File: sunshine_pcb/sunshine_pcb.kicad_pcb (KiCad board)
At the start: 4 copper layers, 30.5 x 44.7 mm, 51 parts, among them J1 VSENS, J2 Conn_01x04, J5 VerticalUSB, Q1 AO3400A, U1 ESP32-S3-WROOM-1, U2 SPX1117M3, U3 LIS3MDL, U4 ADXL375, U8 USBLC6-2P6

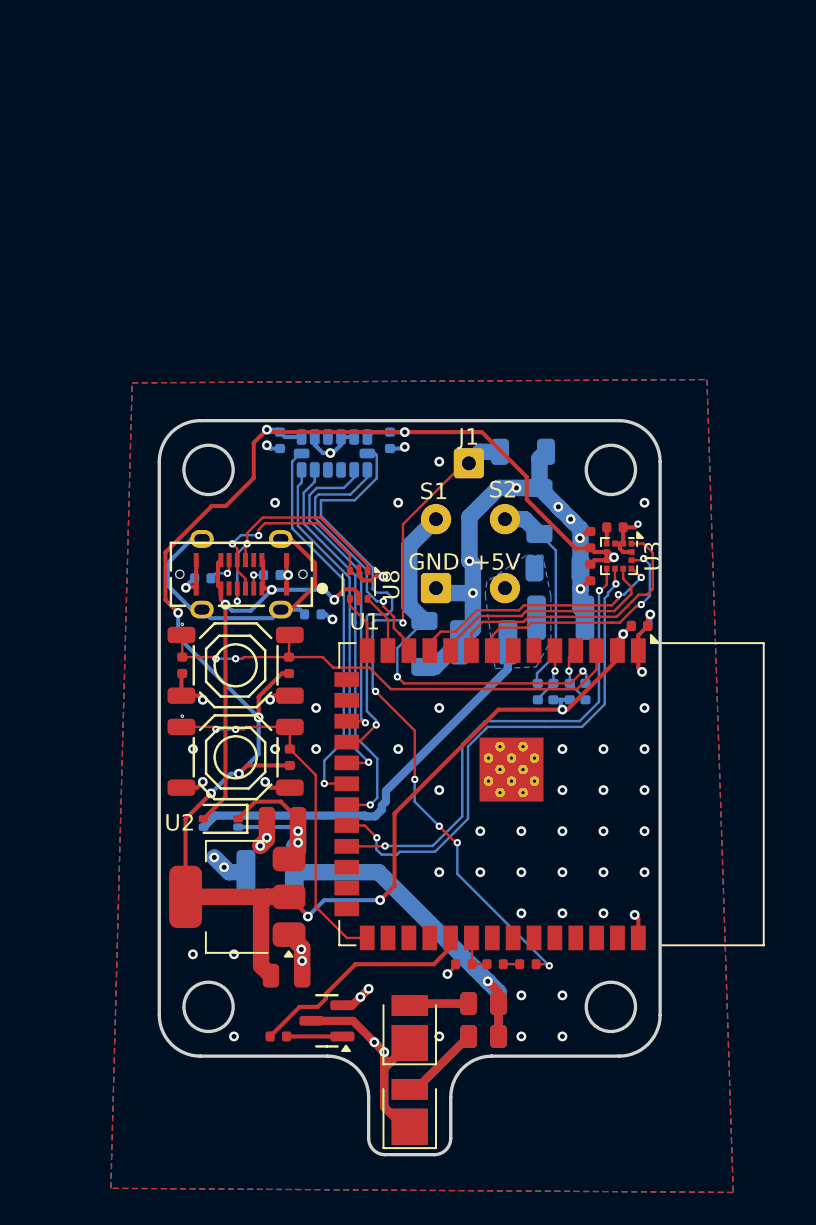
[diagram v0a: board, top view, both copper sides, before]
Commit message: Re-layout PCB
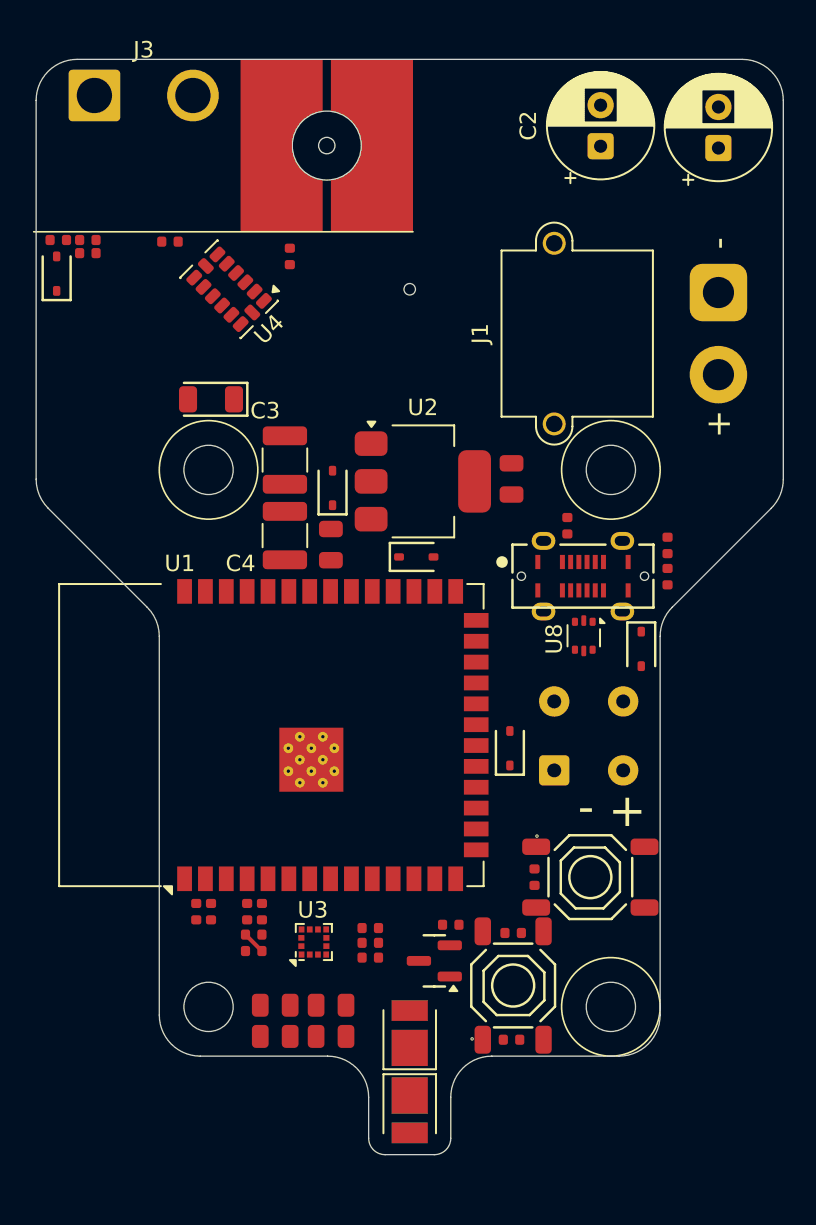
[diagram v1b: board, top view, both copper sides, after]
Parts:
- removed D7: SMF5.0A, PCM_JLCPCB:D_SOD-123FL
- removed R14, R9: 1kΩ, PCM_JLCPCB:R_0402
- added C1: 120u, Capacitor_THT:CP_Radial_D6.3mm_P2.50mm, F.Cu at (118.8, 91.4)
- added D11: H5VLD3B, PCM_JLCPCB:D_SOD-323, F.Cu at (78.5, 99.0)
- added J3: PWROUT, Connector_Wire:SolderWire-1.5sqmm_1x02_P6mm_D1.7mm_OD3mm, F.Cu at (80.8, 88.2)
- added R13: 2kΩ, PCM_JLCPCB:R_0402, F.Cu at (78.6, 97.0)
- added R17: 1kΩ, PCM_JLCPCB:R_0402, F.Cu at (80.4, 97.8)
- added SW1: SW_SPST, custom:screw_switch, F.Cu at (95.0, 91.2)
- C2: value 10u -> 120u; footprint Capacitor_SMD:C_1210_3225Metric -> Capacitor_THT:CP_Radial_D6.3mm_P2.50mm; moved to F.Cu
- C25, C26, C3, C4, C8, D2, D6, D8, R1, R12, R2, R20, R21, R3, R6, R7, R8, U4: moved to F.Cu
- D10, D9: value SMF5.0A -> H5VLD3B; footprint PCM_JLCPCB:D_SOD-123FL -> PCM_JLCPCB:D_SOD-323; moved to F.Cu
- D4: moved to B.Cu
- J1: value VSENS -> PWRIN; footprint Connector_Wire:SolderWire-0.25sqmm_1x01_D0.65mm_OD1.7mm -> Connector_AMASS:AMASS_XT30PW-M_1x02_P2.50mm_Horizontal
- moved R15 49.7 mm to (80.4, 97.0), turned to 0 degrees
- moved C6 33.2 mm to (106.2, 111.5), turned to -90 degrees
- moved C9 32.1 mm to (87.0, 137.9), turned to -90 degrees
- moved C8 31.4 mm to (87.9, 137.9), turned to -90 degrees
- moved C7 30.4 mm to (106.2, 145.7), turned to 0 degrees
- moved C27 30.1 mm to (97.6, 140.7)
- moved U3 30.0 mm to (94.2, 139.8), turned to 90 degrees
- moved C2 28.8 mm to (111.6, 91.3), turned to 90 degrees
- moved R2 28.3 mm to (115.7, 117.5), turned to 90 degrees
- moved C28 28.0 mm to (97.6, 139.8), turned to 0 degrees
- moved U2 27.7 mm to (100.8, 111.7), turned to 0 degrees
- moved S1 25.8 mm to (106.3, 142.4), turned to 90 degrees
- moved C29 25.5 mm to (97.6, 138.9), turned to 0 degrees
- moved R6 24.9 mm to (90.5, 140.3), turned to 180 degrees
- moved R21 24.6 mm to (90.1, 137.9), turned to -90 degrees
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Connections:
- C2 pad 1: /5V_IN -> /BATT+_IN
- C2 pad 2: GND -> /BATT-
- D10 pad 1: /S1_C -> GND
- D10 pad 2: GND -> /S1_C
- D9 pad 1: /S2_C -> GND
- D9 pad 2: GND -> /S2_C
- J1 pad 1: /VSE -> /BATT-
- R15 pad 1: /VSENSE -> /VSE
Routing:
- net +3V3: track 122.6 -> 1.41 mm, vias 11 -> 0
- net GND: track 73.5 -> 0.00 mm, vias 71 -> 0
- net /VSE: track 42.0 -> 0.00 mm, vias 6 -> 0
- net +5V: track 35.3 -> 0.00 mm, vias 3 -> 0
- net /MAG_DRDY: track 31.8 -> 0.00 mm, vias 2 -> 0
- net /EN: track 30.6 -> 0.00 mm, vias 2 -> 0
- net /MAG_INT: track 29.9 -> 0.00 mm, vias 2 -> 0
- net VBUS: track 29.2 -> 0.00 mm, vias 3 -> 0
- net /IMU_CS: track 25.6 -> 0.00 mm, vias 1 -> 0
- net /5V_IN: track 24.7 -> 0.00 mm
- net /IMU_MISO: track 24.3 -> 0.00 mm, vias 1 -> 0
- net /S1_C: track 23.9 -> 0.00 mm, vias 2 -> 0
- net /IMU_SCK: track 23.5 -> 0.00 mm, vias 1 -> 0
- net /BOOT: track 22.4 -> 0.00 mm, vias 2 -> 0
- net Net-(D1-K): track 21.2 -> 0.00 mm, vias 2 -> 0
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- removed copper zone on B.Cu, net /5V_IN
- removed copper zone on B.Cu, net GND
- removed copper zone on F.Cu, net GND
- removed copper zone on In1.Cu, net GND
- removed copper zone on In2.Cu, net GND
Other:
- board size 30.5 x 44.7 mm -> 45.5 x 66.7 mm
- board text added: "+ -"
- board text removed: "+5V"
- board text removed: "GND"
- board text removed: "S1"
- board text removed: "S2"
